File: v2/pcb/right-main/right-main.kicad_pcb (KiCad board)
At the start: 2 copper layers, 83 x 79 mm, 33 parts, among them J1 Conn_01x10, SW1 SW_Push, SW10 SW_Push, SW11 SW_Push, SW12 SW_Push, SW13 SW_Push, SW14 SW_Push, SW15 SW_Push, SW16 SW_Push, SW2 SW_Push, SW3 SW_Push, SW4 SW_Push, SW5 SW_Push, SW6 SW_Push, SW7 SW_Push, SW8 SW_Push, SW9 SW_Push

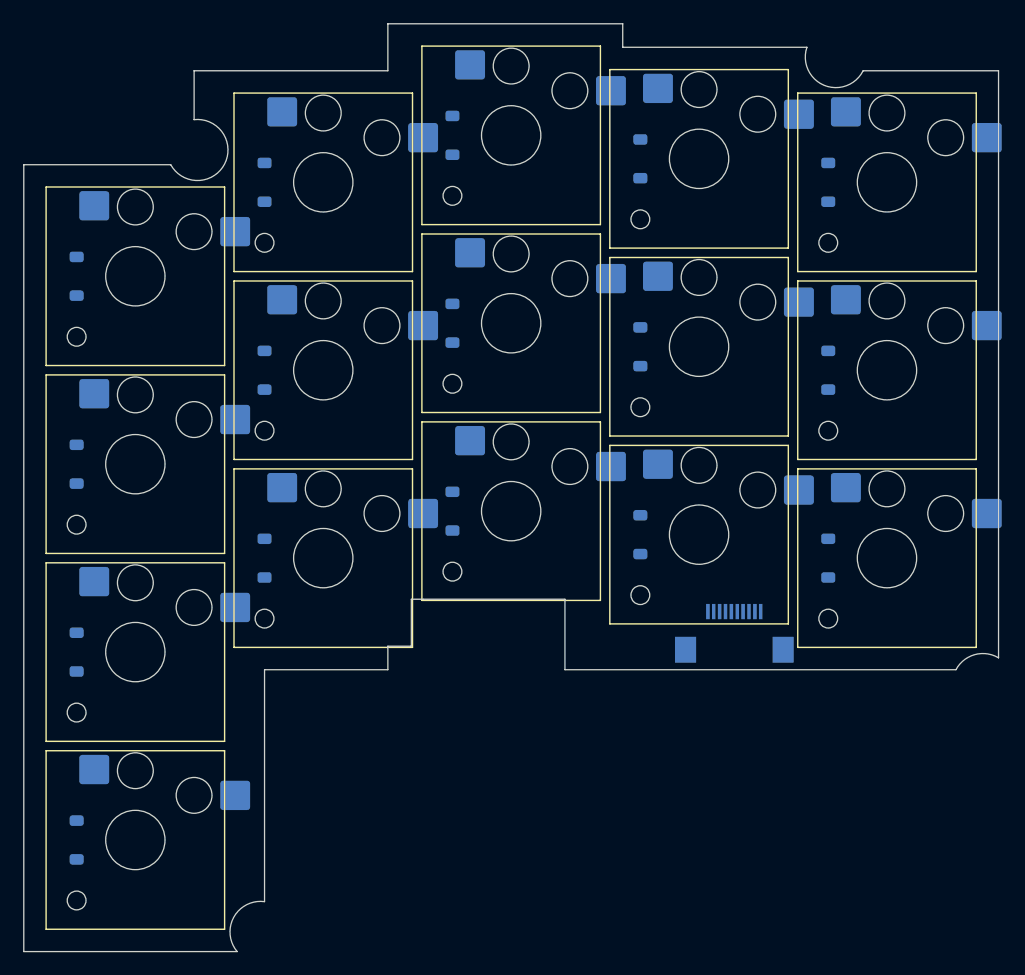
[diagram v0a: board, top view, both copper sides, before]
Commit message: feat: update case data
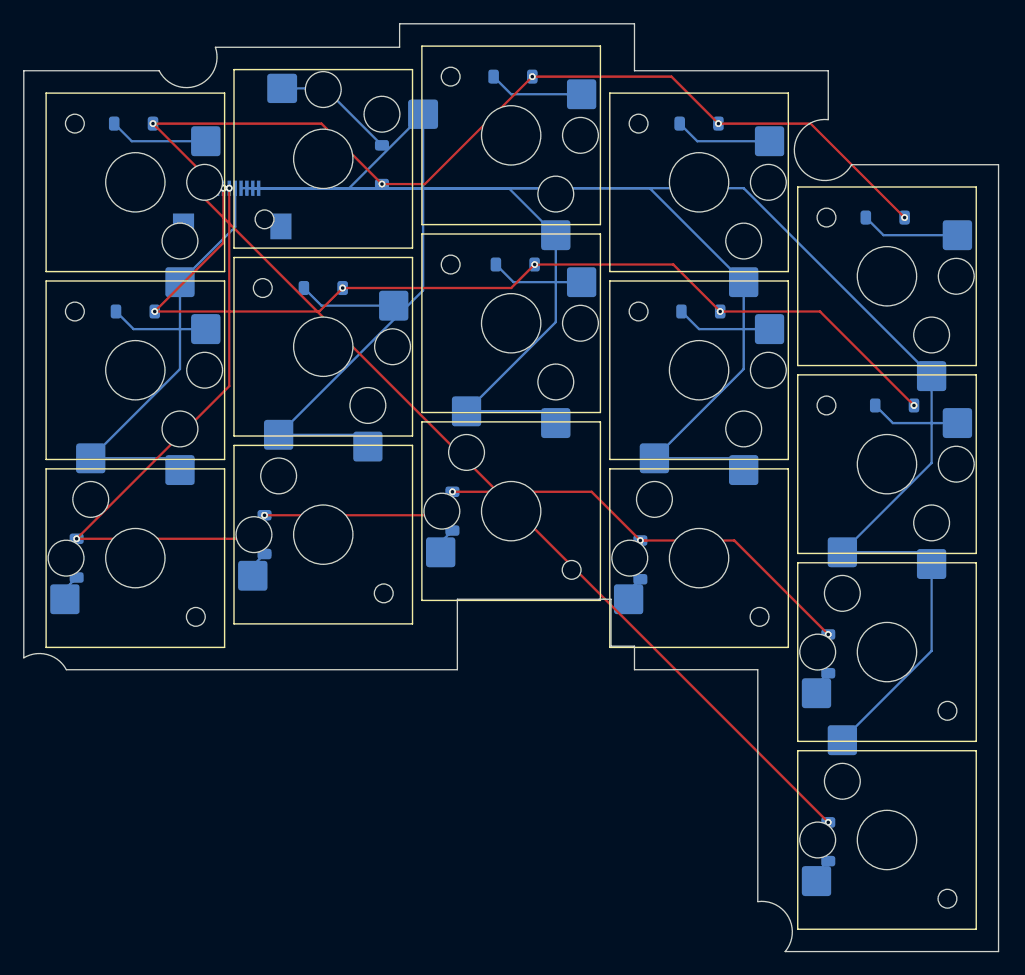
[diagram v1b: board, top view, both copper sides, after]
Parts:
- moved D10 69.8 mm to (198.7, 110.5), turned to 0 degrees
- moved D5 69.0 mm to (197.8, 94.5), turned to 0 degrees
- moved D15 64.0 mm to (193.0, 131.7), turned to 90 degrees
- moved D16 64.0 mm to (193.0, 147.7), turned to 90 degrees
- moved D11 64.0 mm to (129.0, 123.5), turned to 90 degrees
- moved SW1 64.0 mm to (134.0, 91.5), turned to -90 degrees
- moved SW10 64.0 mm to (198.0, 115.5), turned to -90 degrees
- moved SW11 64.0 mm to (134.0, 123.5), turned to 90 degrees
- moved SW15 64.0 mm to (198.0, 131.5), turned to 90 degrees
- moved SW16 64.0 mm to (198.0, 147.5), turned to 90 degrees
- moved SW5 64.0 mm to (198.0, 99.5), turned to -90 degrees
- moved SW6 64.0 mm to (134.0, 107.5), turned to -90 degrees
- moved D1 59.4 mm to (133.8, 86.5), turned to 0 degrees
- moved D6 59.2 mm to (134.0, 102.5), turned to 0 degrees
- moved J1 55.9 mm to (142.2, 93.8)
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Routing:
- net /COL4: track 0.00 -> 108.2 mm
- net /ROW2: track 0.00 -> 105.9 mm, vias 0 -> 6
- net /ROW1: track 0.00 -> 84.2 mm, vias 0 -> 6
- net /ROW0: track 0.00 -> 82.7 mm, vias 0 -> 6
- net /ROW3: track 0.00 -> 76.0 mm, vias 0 -> 2
- net /COL3: track 0.00 -> 71.3 mm
- net /COL1: track 0.00 -> 58.5 mm
- net /COL2: track 0.00 -> 54.1 mm
- net /COL0: track 0.00 -> 36.1 mm
- net Net-(D2-K): track 0.00 -> 10.5 mm
- net Net-(D1-K): track 0.00 -> 8.42 mm
- net Net-(D5-K): track 0.00 -> 8.42 mm
- net Net-(D7-K): track 0.00 -> 8.27 mm
- net Net-(D6-K): track 0.00 -> 8.27 mm
- net Net-(D4-K): track 0.00 -> 8.27 mm
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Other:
- outline, holes or cut-outs redrawn
